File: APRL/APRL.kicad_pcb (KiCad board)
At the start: 2 copper layers, 1 part, among them U1 BMP581

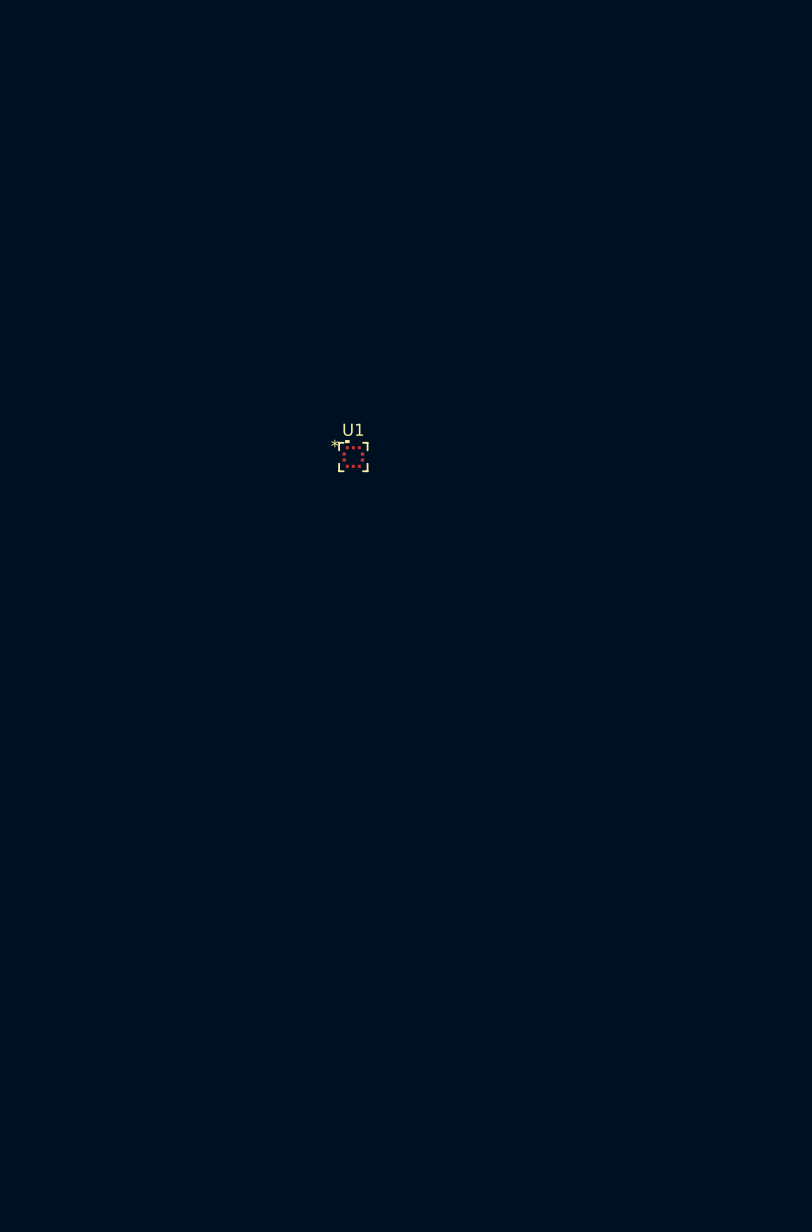
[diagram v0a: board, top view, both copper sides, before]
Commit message: schematics
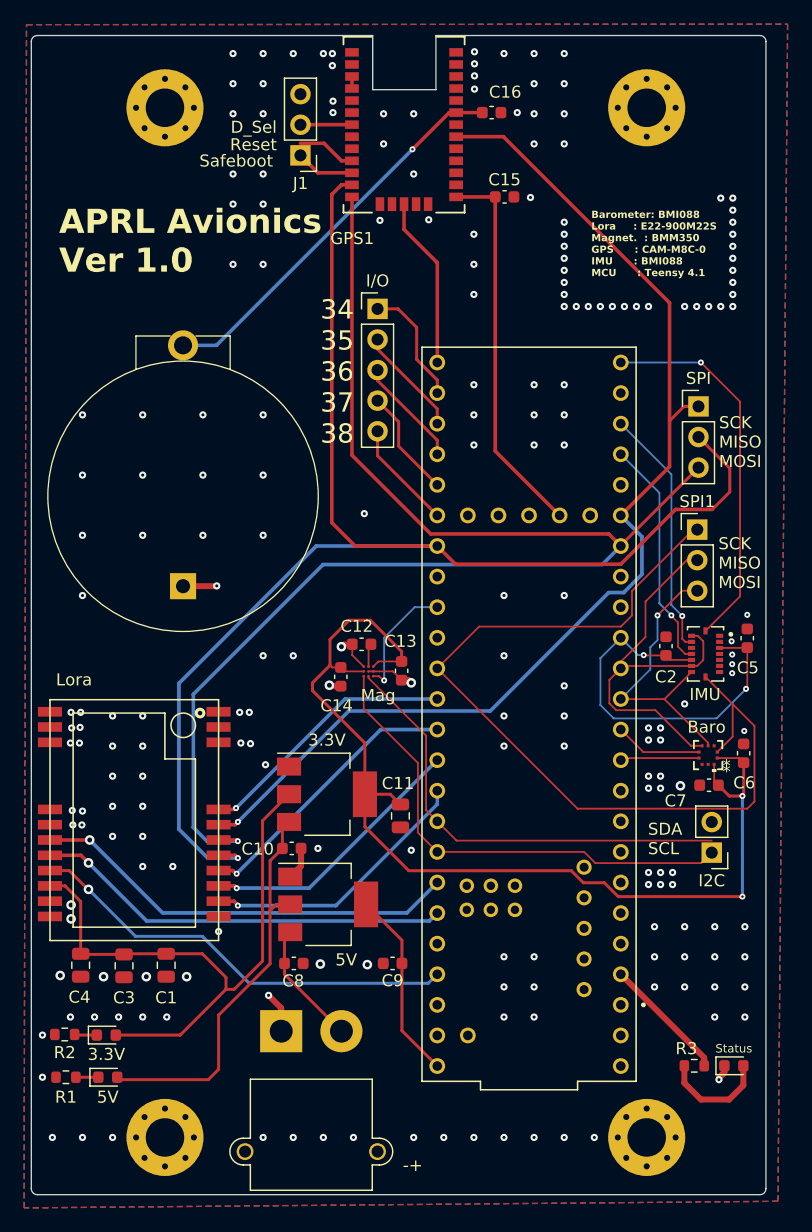
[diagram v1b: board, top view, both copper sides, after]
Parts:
- removed U1: BMP581, footprints:QFN10_BMP581_BOS
- added 3.3V: AP1117-15, Package_TO_SOT_SMD:SOT-223-3_TabPin2, F.Cu at (140.3, 111.5)
- added 3.3V: LED, LED_SMD:LED_0603_1608Metric, F.Cu at (122.0, 131.5)
- added 5V: AP1117-50, Package_TO_SOT_SMD:SOT-223-3_TabPin2, F.Cu at (140.4, 120.7)
- added 5V: LED, LED_SMD:LED_0603_1608Metric, F.Cu at (122.1, 135.0)
- added BAT1: BS-7, footprints:Battery_Holder_Coin_2032_BS-7, F.Cu at (128.3, 94.2)
- added BT1: 2S, footprints:AMASS_XT30PW-M_1x02_P2.50mm_Horizontal, F.Cu at (136.5, 131.2)
- added Baro: BMP581, footprints:QFN10_BMP581_BOS, F.Cu at (171.9, 108.2)
- added C1: 22uF, Capacitor_SMD:C_0805_2012Metric, F.Cu at (127.0, 125.7)
- added C10: 10uF, Capacitor_SMD:C_0603_1608Metric, F.Cu at (137.4, 116.0)
- added C11: 100uF, Capacitor_SMD:C_0805_2012Metric, F.Cu at (146.4, 113.3)
- added C12: 2.2uF, Capacitor_SMD:C_0603_1608Metric, F.Cu at (143.2, 99.0)
- added C13: 100nF, Capacitor_SMD:C_0603_1608Metric, F.Cu at (146.5, 101.2)
- added C14: 100nF, Capacitor_SMD:C_0603_1608Metric, F.Cu at (141.4, 101.8)
- added C15: 4.7 uF, Capacitor_SMD:C_0603_1608Metric, F.Cu at (155.1, 61.9)
- added C16: 100nF, Capacitor_SMD:C_0603_1608Metric, F.Cu at (154.0, 54.9)
- added C2: 100nF, Capacitor_SMD:C_0603_1608Metric, F.Cu at (168.4, 99.2)
- added C3: 10uF, Capacitor_SMD:C_0805_2012Metric, F.Cu at (123.5, 125.8)
- added C4: 100nF, Capacitor_SMD:C_0805_2012Metric, F.Cu at (119.8, 125.7)
- added C5: 100nF, Capacitor_SMD:C_0603_1608Metric, F.Cu at (175.2, 98.5)
- added C6: 100nF, Capacitor_SMD:C_0603_1608Metric, F.Cu at (174.9, 108.1)
- added C7: 100nF, Capacitor_SMD:C_0603_1608Metric, F.Cu at (172.0, 110.8)
- added C8: 1 uF, Capacitor_SMD:C_0603_1608Metric, F.Cu at (137.6, 125.5)
- added C9: 100 nF, Capacitor_SMD:C_0603_1608Metric, F.Cu at (145.8, 125.5)
- added G***: LOGO, LOGO, B.Cu at (126.8, 64.6)
- added G***: LOGO, LOGO, B.Cu at (165.5, 67.6)
- added GPS1: CAM-M8C-0, footprints:QFN_M8C-0_UBL, F.Cu at (146.7, 55.9)
- added I/O: Conn_01x05_Pin, Connector_PinHeader_2.54mm:PinHeader_1x05_P2.54mm_Vertical, F.Cu at (144.5, 71.2)
- added I2C: Conn_01x02_Pin, Connector_PinHeader_2.54mm:PinHeader_1x02_P2.54mm_Vertical, F.Cu at (172.2, 116.3)
- added IMU: BMI088, footprints:PQFN50P450X300X100-16N, F.Cu at (171.7, 99.8)
- added J1: Conn_01x03_Pin, Connector_PinHeader_2.54mm:PinHeader_1x03_P2.54mm_Vertical, F.Cu at (138.1, 58.5)
- added Lora: E22-900M22S, footprints:E22-900M22S, F.Cu at (124.3, 113.7)
- added MCU1: Teensy 4.1, footprints:Teensy_41, F.Cu at (157.1, 104.9)
- added Mag: BMM350, footprints:BGA9_BMM350_BOS, F.Cu at (143.7, 101.3)
- added R1: 1k, Resistor_SMD:R_0603_1608Metric, F.Cu at (118.6, 135.0)
- added R2: 1k, Resistor_SMD:R_0603_1608Metric, F.Cu at (118.5, 131.4)
- added R3: 1k, Resistor_SMD:R_0603_1608Metric, F.Cu at (170.8, 134.1)
- added REF**: MountingHole_3.2mm_M3_Pad_Via, MountingHole:MountingHole_3.2mm_M3_Pad_Via, F.Cu at (126.8, 54.5)
- added REF**: MountingHole_3.2mm_M3_Pad_Via, MountingHole:MountingHole_3.2mm_M3_Pad_Via, F.Cu at (126.8, 140.0)
- added REF**: MountingHole_3.2mm_M3_Pad_Via, MountingHole:MountingHole_3.2mm_M3_Pad_Via, F.Cu at (166.8, 54.5)
- added REF**: MountingHole_3.2mm_M3_Pad_Via, MountingHole:MountingHole_3.2mm_M3_Pad_Via, F.Cu at (166.8, 140.0)
- added SPI: Conn_01x03_Pin, Connector_PinHeader_2.54mm:PinHeader_1x03_P2.54mm_Vertical, F.Cu at (171.2, 79.3)
- added SPI1: Conn_01x03_Pin, Connector_PinHeader_2.54mm:PinHeader_1x03_P2.54mm_Vertical, F.Cu at (171.1, 89.5)
- added Status: LED, LED_SMD:LED_0603_1608Metric, F.Cu at (174.1, 134.1)
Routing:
- net +3.3V: track 0.00 -> 202.1 mm, vias 0 -> 4
- net SPI_MISO1: track 0.00 -> 117.7 mm, vias 0 -> 1
- net SPI_MOSI1: track 0.00 -> 113.7 mm, vias 0 -> 1
- net SPI_SCK1: track 0.00 -> 95.1 mm, vias 0 -> 1
- net SPI_SCK: track 0.00 -> 76.0 mm
- net +5V: track 0.00 -> 49.6 mm
- net SCL: track 0.00 -> 40.7 mm
- net SDA: track 0.00 -> 37.9 mm
- net /DIO2: track 0.00 -> 36.5 mm, vias 0 -> 1
- net RXEN: track 0.00 -> 35.7 mm, vias 0 -> 1
- net SPI_MISO: track 0.00 -> 34.9 mm
- net TXEN: track 0.00 -> 34.7 mm, vias 0 -> 1
- net Net-(GPS1-V_BCKP): track 0.00 -> 32.9 mm, vias 0 -> 1
- net IMU_INT1: track 0.00 -> 31.5 mm, vias 0 -> 1
- net SPI_MOSI: track 0.00 -> 25.0 mm, vias 0 -> 1
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- added copper zone on B.Cu, net GND
- added copper zone on F.Cu, net GND
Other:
- board outline added: 61 x 96.2 mm
- board text added: "-+"
- board text added: "34 35 36 37 38"
- board text added: "APRL Avionics Ver 1.0"
- board text added: "APRL Gliding Beaver"
- board text added: "Barometer: BMI088 Lora : E22-900M22S Magnet. : BMM350 GPS : CAM-M8C-0 IMU : BMI088 MCU : Teensy 4.1"
- board text added: "D_Sel"
- board text added: "IMU"
- board text added: "Reset"
- board text added: "SCK MISO MOSI"
- board text added: "SDA SCL"
- board text added: "Safeboot"
